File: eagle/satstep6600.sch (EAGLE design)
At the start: 42 parts, among them J3 STEPPER_CONN_2, T1 5K, U1 74HC123D

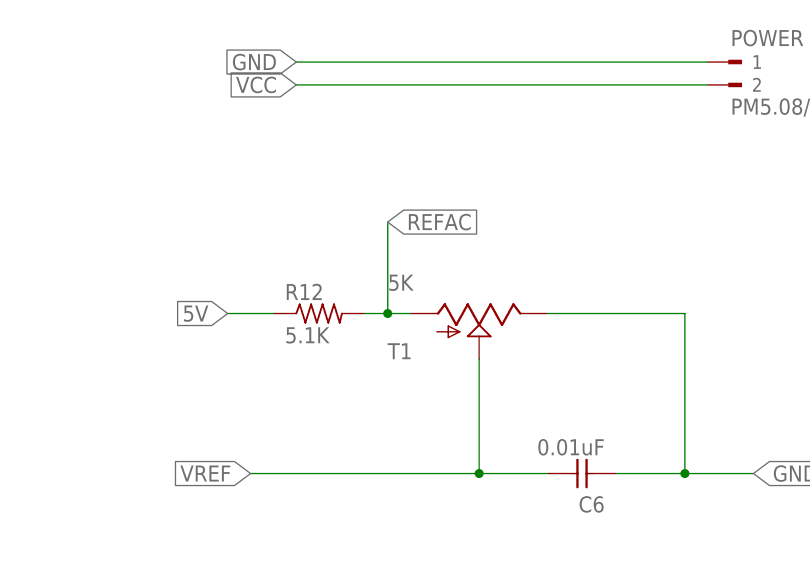
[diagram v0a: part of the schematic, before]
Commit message: safier trimmer value
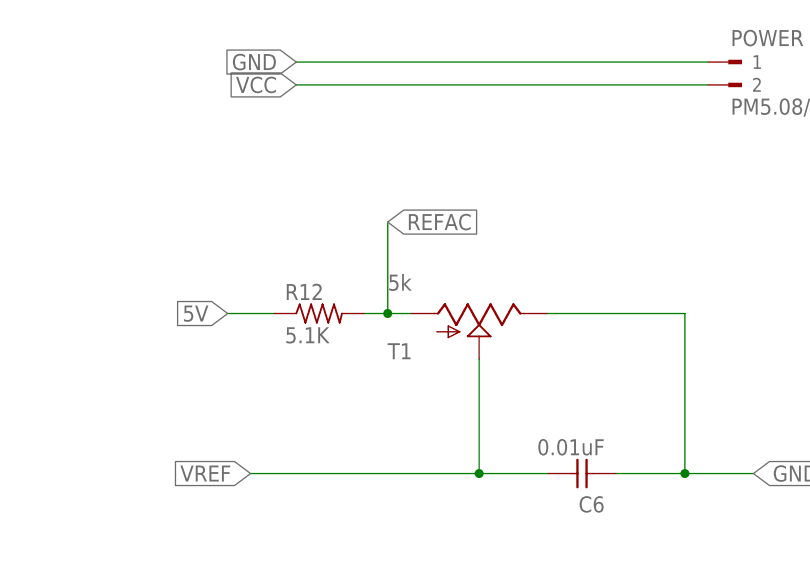
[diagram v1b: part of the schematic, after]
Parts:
- T1: value 5K -> 5k
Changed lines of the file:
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@@
 <part name="C6" library="FAB_Hello" deviceset="UNPOLARIZED_CAPACITOR" device="1206" value="0.01uF"/>
 <part name="R12" library="fab" deviceset="RES-US" device="1206" value="5.1K"/>
-<part name="T1" library="Ava" deviceset="TS53YL104MR10-TRIMMER" device="" value="5K"/>
+<part name="T1" library="Ava" deviceset="TS53YL104MR10-TRIMMER" device="" value="5k"/>
 <part name="U1" library="74HC123D" deviceset="74HC123D" device=""/>
 <part name="R13" library="fab" deviceset="RES-US" device="1206" value="5.1K"/>
